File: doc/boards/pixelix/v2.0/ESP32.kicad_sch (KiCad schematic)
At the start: 2 parts, among them U1 ESP32-DEVKITC-32D

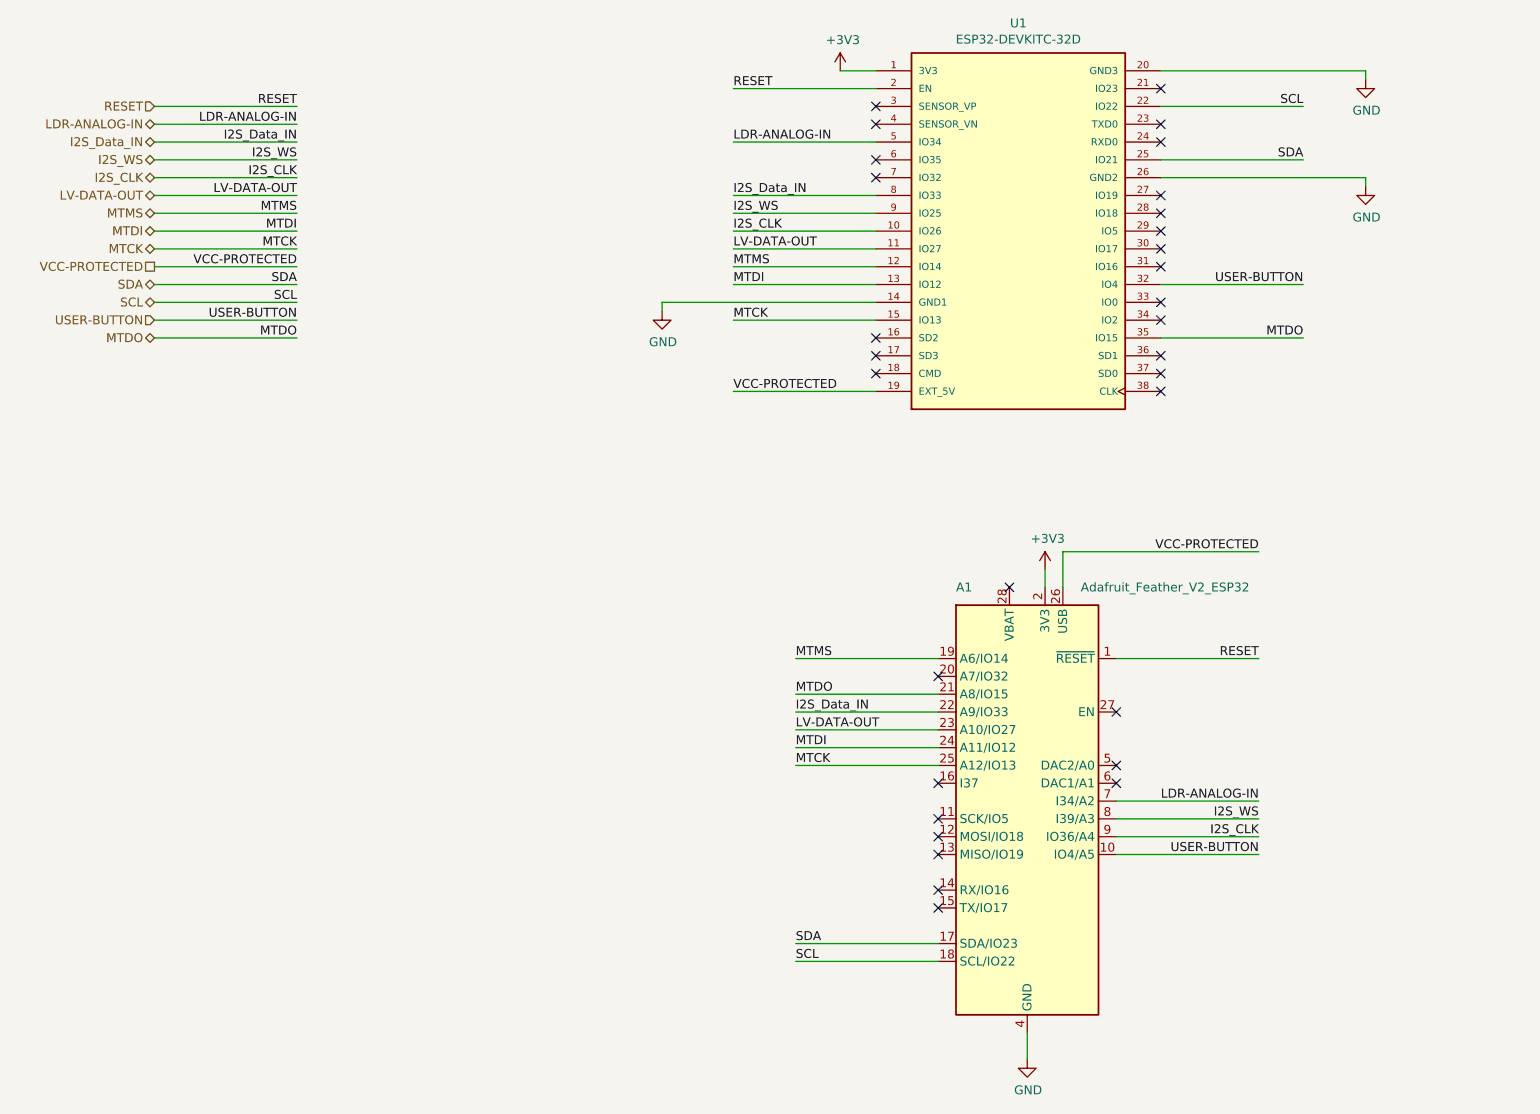
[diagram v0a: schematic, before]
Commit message: #91 Board v2.1 Schmatic - I2S Pins on Feather updated (see Table: https://github.com/BlueAndi/esp-rgb-led-matrix/blob/Development/doc/boards/pixelix/v2.0/ELECTRONIC.md)
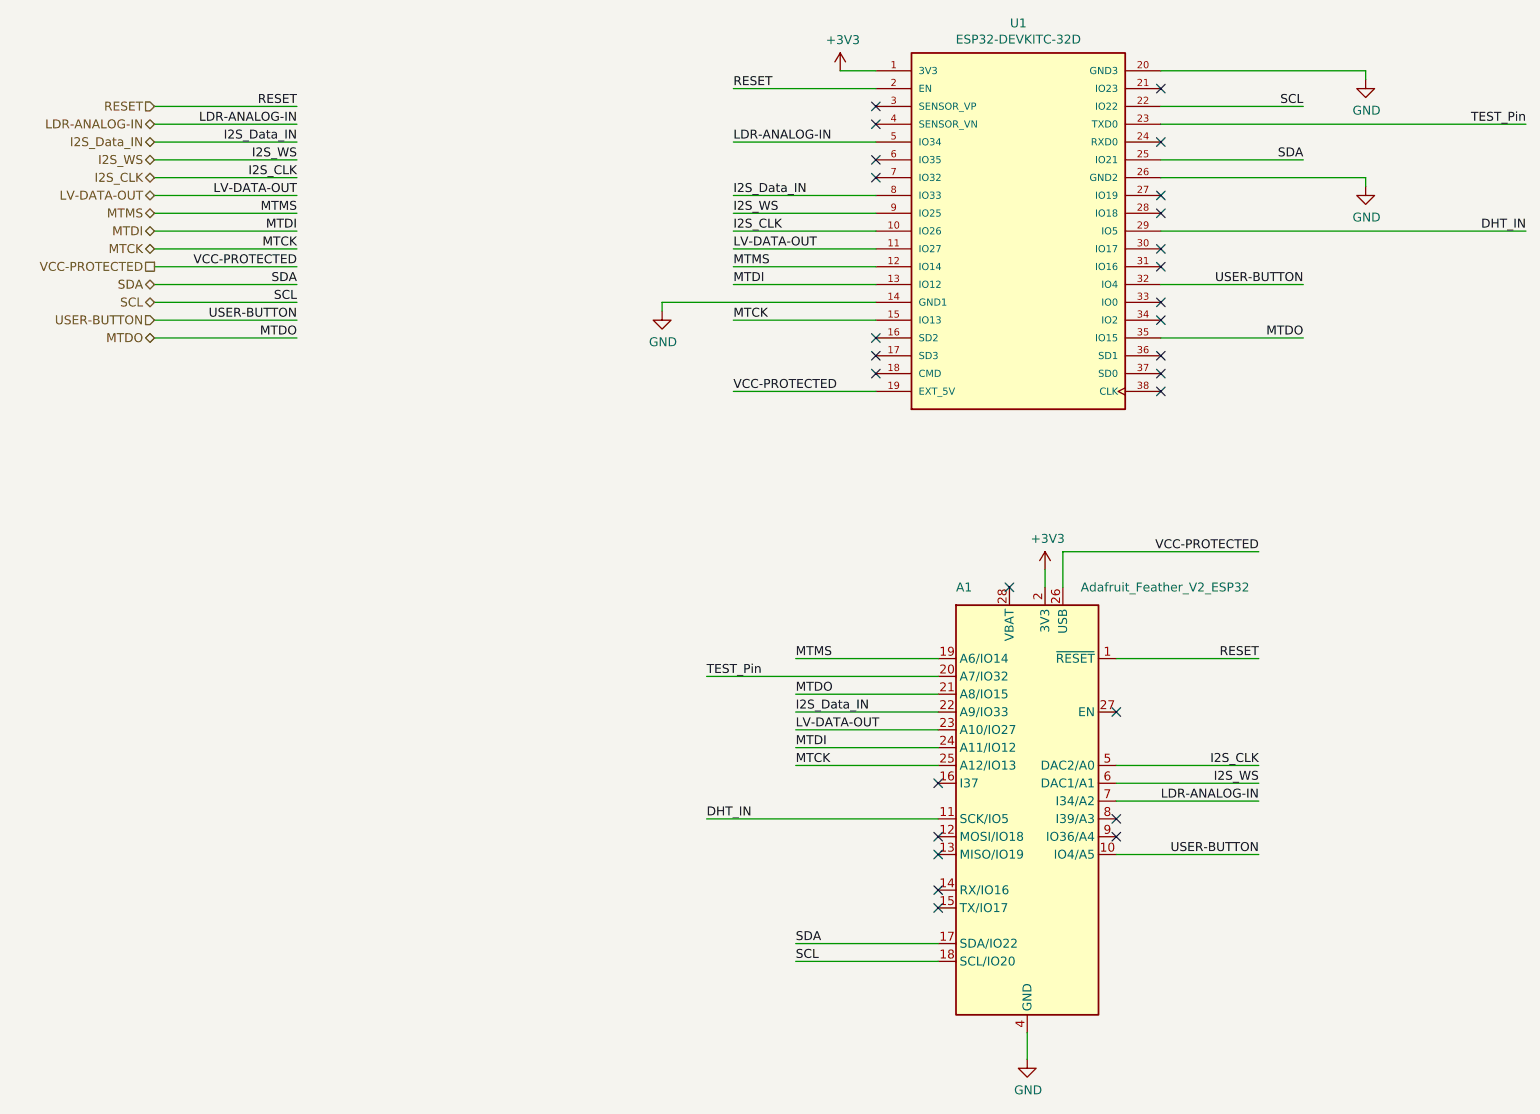
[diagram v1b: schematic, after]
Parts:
- A1: footprint footprints:Adafruit_Feather_V2_ESP32 -> Module:Adafruit_Feather
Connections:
- net I2S_CLK: now also A1.5 (DAC2/A0); no longer A1.9 (IO36/A4)
- net I2S_WS: now also A1.6 (DAC1/A1); no longer A1.8 (I39/A3)
- net TEST_Pin: now reaches U1.23 (TXD0)
- net TEST_Pin: now also A1.20 (A7/IO32)
- net DHT_IN: now reaches U1.29 (IO5)
- net DHT_IN: now also A1.11 (SCK/IO5)
- no-connect marks 31 -> 27
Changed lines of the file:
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@@
   (no_connect (at 139.7 30.48))
   (no_connect (at 180.34 66.04))
-  (no_connect (at 173.99 121.92))
-  (no_connect (at 173.99 124.46))
+  (no_connect (at 173.99 129.54))
+  (no_connect (at 173.99 132.08))
   (no_connect (at 180.34 55.88))
   (no_connect (at 139.7 60.96))
-  (no_connect (at 180.34 30.48))
   (no_connect (at 139.7 63.5))
   (no_connect (at 139.7 27.94))
   (no_connect (at 139.7 35.56))
-  (no_connect (at 148.59 109.22))
   (no_connect (at 180.34 48.26))
   (no_connect (at 148.59 124.46))
-  (no_connect (at 180.34 45.72))
   (no_connect (at 148.59 134.62))
-  (no_connect (at 148.59 129.54))
   (no_connect (at 148.59 142.24))
   (no_connect (at 180.34 43.18))
@@
     (stroke (width 0) (type default) (color 0 0 0 0))
   )
-  (wire (pts (xy 194.31 132.08) (xy 173.99 132.08))
+  (wire (pts (xy 194.31 121.92) (xy 173.99 121.92))
     (stroke (width 0) (type default) (color 0 0 0 0))
   )
@@
     (stroke (width 0) (type default) (color 0 0 0 0))
   )
+  (wire (pts (xy 115.57 129.54) (xy 148.59 129.54))
+    (stroke (width 0) (type default) (color 0 0 0 0))
+  )
+  (wire (pts (xy 115.57 109.22) (xy 148.59 109.22))
+    (stroke (width 0) (type default) (color 0 0 0 0))
+  )
   (wire (pts (xy 209.55 22.86) (xy 180.34 22.86))
     (stroke (width 0) (type default) (color 0 0 0 0))
@@
     (stroke (width 0) (type default) (color 0 0 0 0))
   )
-  (wire (pts (xy 194.31 129.54) (xy 173.99 129.54))
+  (wire (pts (xy 180.34 45.72) (xy 232.41 45.72))
+    (stroke (width 0) (type default) (color 0 0 0 0))
+  )
+  (wire (pts (xy 194.31 124.46) (xy 173.99 124.46))
+    (stroke (width 0) (type default) (color 0 0 0 0))
+  )
+  (wire (pts (xy 232.41 30.48) (xy 180.34 30.48))
     (stroke (width 0) (type default) (color 0 0 0 0))
   )
@@
     (effects (font (size 1.27 1.27)) (justify left bottom))
   )
-  (label "I2S_CLK" (at 194.31 132.08 180)
+  (label "I2S_CLK" (at 194.31 121.92 180)
     (effects (font (size 1.27 1.27)) (justify right bottom))
   )
@@
     (effects (font (size 1.27 1.27)) (justify left bottom))
   )
+  (label "TEST_Pin" (at 115.57 109.22 0)
+    (effects (font (size 1.27 1.27)) (justify left bottom))
+  )
   (label "LDR-ANALOG-IN" (at 57.15 30.48 180)
     (effects (font (size 1.27 1.27)) (justify right bottom))
   )
+  (label "DHT_IN" (at 232.41 45.72 180)
+    (effects (font (size 1.27 1.27)) (justify right bottom))
+  )
   (label "SDA" (at 128.27 147.32 0)
     (effects (font (size 1.27 1.27)) (justify left bottom))
@@
     (effects (font (size 1.27 1.27)) (justify right bottom))
   )
+  (label "TEST_Pin" (at 232.41 30.48 180)
+    (effects (font (size 1.27 1.27)) (justify right bottom))
+  )
   (label "MTCK" (at 119.38 58.42 0)
     (effects (font (size 1.27 1.27)) (justify left bottom))
@@
     (effects (font (size 1.27 1.27)) (justify right bottom))
   )
-  (label "I2S_WS" (at 194.31 129.54 180)
+  (label "I2S_WS" (at 194.31 124.46 180)
     (effects (font (size 1.27 1.27)) (justify right bottom))
   )
@@
   )
   (label "SCL" (at 128.27 149.86 0)
+    (effects (font (size 1.27 1.27)) (justify left bottom))
+  )
+  (label "DHT_IN" (at 115.57 129.54 0)
     (effects (font (size 1.27 1.27)) (justify left bottom))
   )
@@
       (effects (font (size 1.27 1.27)) (justify left))
     )
-    (property "Footprint" "footprints:Adafruit_Feather_V2_ESP32" (id 2) (at 163.83 161.29 0)
+    (property "Footprint" "Module:Adafruit_Feather" (id 2) (at 163.83 161.29 0)
       (effects (font (size 1.27 1.27)) (justify left) hide)
     )

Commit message: Revert "#91 Board v2.1 Schmatic"
This reverts commit 70677a910b1cfea4215dbaf6ed272a144c07ba06.
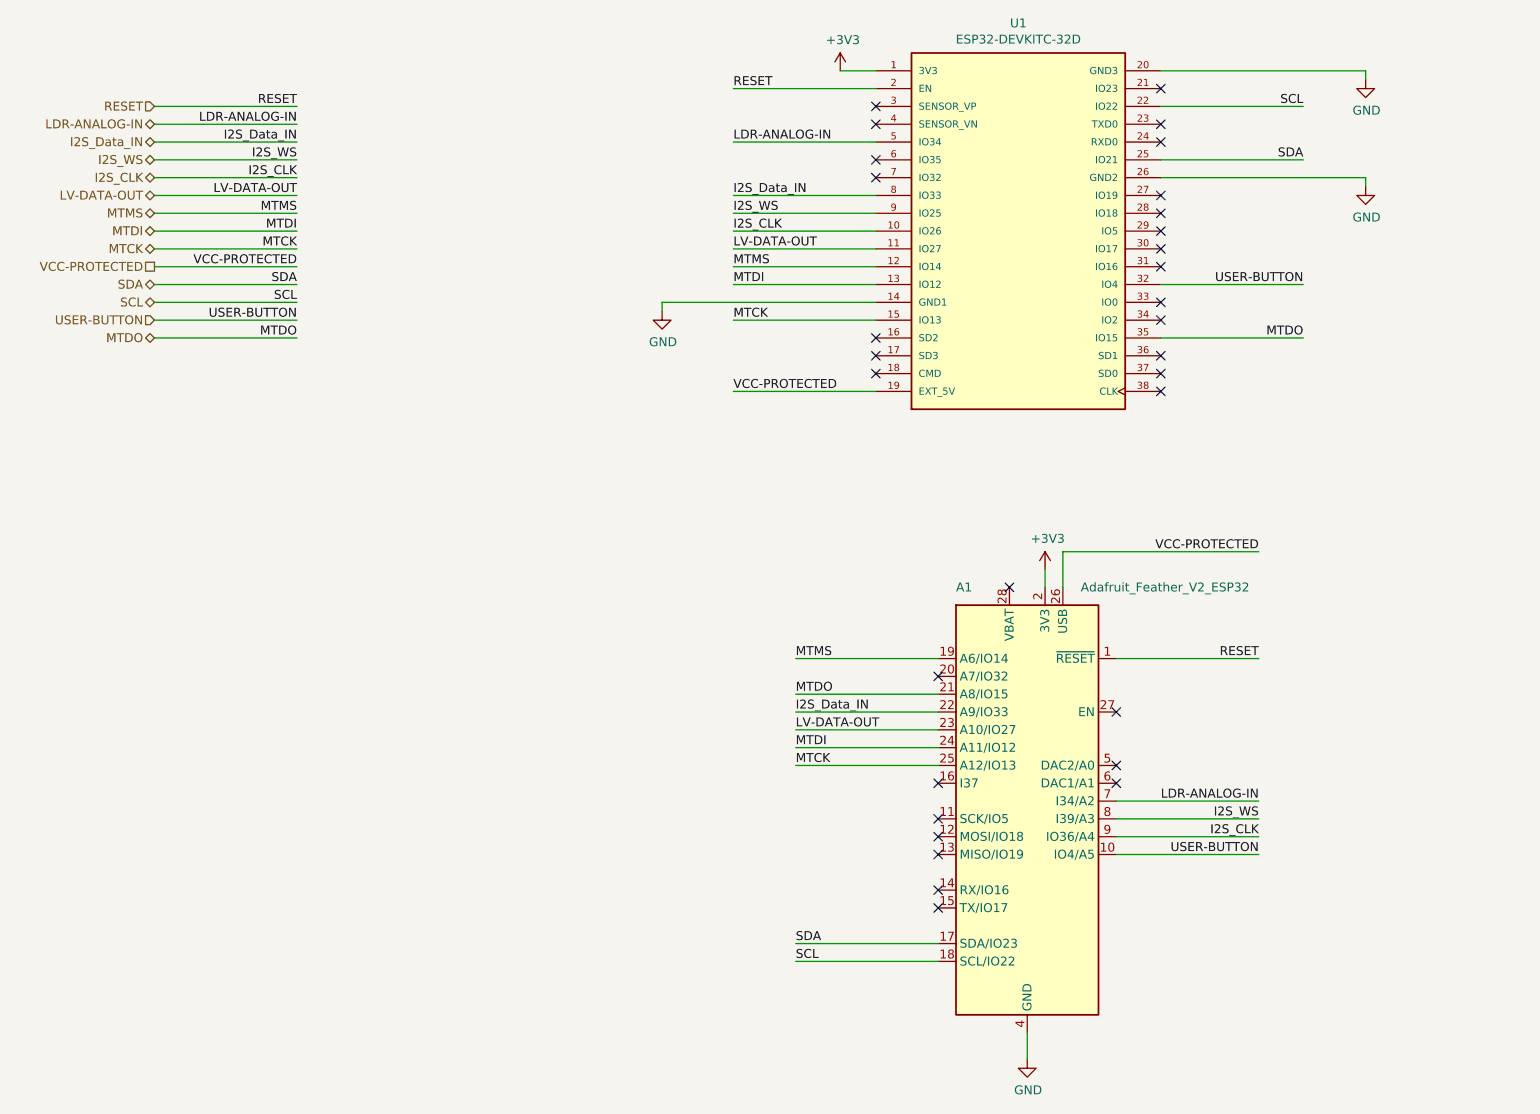
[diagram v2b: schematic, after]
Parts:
- A1: footprint Module:Adafruit_Feather -> footprints:Adafruit_Feather_V2_ESP32
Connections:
- net I2S_CLK: now also A1.9 (IO36/A4); no longer A1.5 (DAC2/A0)
- net I2S_WS: now also A1.8 (I39/A3); no longer A1.6 (DAC1/A1)
- net DHT_IN: no longer names the net of U1.29 (IO5)
- net DHT_IN: no longer A1.11 (SCK/IO5)
- net TEST_Pin: no longer names the net of U1.23 (TXD0)
- net TEST_Pin: no longer A1.20 (A7/IO32)
- no-connect marks 27 -> 31
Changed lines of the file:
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@@
   (no_connect (at 139.7 30.48))
   (no_connect (at 180.34 66.04))
-  (no_connect (at 173.99 129.54))
-  (no_connect (at 173.99 132.08))
+  (no_connect (at 173.99 121.92))
+  (no_connect (at 173.99 124.46))
   (no_connect (at 180.34 55.88))
   (no_connect (at 139.7 60.96))
+  (no_connect (at 180.34 30.48))
   (no_connect (at 139.7 63.5))
   (no_connect (at 139.7 27.94))
   (no_connect (at 139.7 35.56))
+  (no_connect (at 148.59 109.22))
   (no_connect (at 180.34 48.26))
   (no_connect (at 148.59 124.46))
+  (no_connect (at 180.34 45.72))
   (no_connect (at 148.59 134.62))
+  (no_connect (at 148.59 129.54))
   (no_connect (at 148.59 142.24))
   (no_connect (at 180.34 43.18))
@@
     (stroke (width 0) (type default) (color 0 0 0 0))
   )
-  (wire (pts (xy 194.31 121.92) (xy 173.99 121.92))
+  (wire (pts (xy 194.31 132.08) (xy 173.99 132.08))
     (stroke (width 0) (type default) (color 0 0 0 0))
   )
@@
     (stroke (width 0) (type default) (color 0 0 0 0))
   )
-  (wire (pts (xy 115.57 129.54) (xy 148.59 129.54))
-    (stroke (width 0) (type default) (color 0 0 0 0))
-  )
-  (wire (pts (xy 115.57 109.22) (xy 148.59 109.22))
-    (stroke (width 0) (type default) (color 0 0 0 0))
-  )
   (wire (pts (xy 209.55 22.86) (xy 180.34 22.86))
     (stroke (width 0) (type default) (color 0 0 0 0))
@@
     (stroke (width 0) (type default) (color 0 0 0 0))
   )
-  (wire (pts (xy 180.34 45.72) (xy 232.41 45.72))
-    (stroke (width 0) (type default) (color 0 0 0 0))
-  )
-  (wire (pts (xy 194.31 124.46) (xy 173.99 124.46))
-    (stroke (width 0) (type default) (color 0 0 0 0))
-  )
-  (wire (pts (xy 232.41 30.48) (xy 180.34 30.48))
+  (wire (pts (xy 194.31 129.54) (xy 173.99 129.54))
     (stroke (width 0) (type default) (color 0 0 0 0))
   )
@@
     (effects (font (size 1.27 1.27)) (justify left bottom))
   )
-  (label "I2S_CLK" (at 194.31 121.92 180)
+  (label "I2S_CLK" (at 194.31 132.08 180)
     (effects (font (size 1.27 1.27)) (justify right bottom))
   )
@@
     (effects (font (size 1.27 1.27)) (justify left bottom))
   )
-  (label "TEST_Pin" (at 115.57 109.22 0)
-    (effects (font (size 1.27 1.27)) (justify left bottom))
-  )
   (label "LDR-ANALOG-IN" (at 57.15 30.48 180)
     (effects (font (size 1.27 1.27)) (justify right bottom))
   )
-  (label "DHT_IN" (at 232.41 45.72 180)
-    (effects (font (size 1.27 1.27)) (justify right bottom))
-  )
   (label "SDA" (at 128.27 147.32 0)
     (effects (font (size 1.27 1.27)) (justify left bottom))
@@
     (effects (font (size 1.27 1.27)) (justify right bottom))
   )
-  (label "TEST_Pin" (at 232.41 30.48 180)
-    (effects (font (size 1.27 1.27)) (justify right bottom))
-  )
   (label "MTCK" (at 119.38 58.42 0)
     (effects (font (size 1.27 1.27)) (justify left bottom))
@@
     (effects (font (size 1.27 1.27)) (justify right bottom))
   )
-  (label "I2S_WS" (at 194.31 124.46 180)
+  (label "I2S_WS" (at 194.31 129.54 180)
     (effects (font (size 1.27 1.27)) (justify right bottom))
   )
@@
   )
   (label "SCL" (at 128.27 149.86 0)
-    (effects (font (size 1.27 1.27)) (justify left bottom))
-  )
-  (label "DHT_IN" (at 115.57 129.54 0)
     (effects (font (size 1.27 1.27)) (justify left bottom))
   )
@@
       (effects (font (size 1.27 1.27)) (justify left))
     )
-    (property "Footprint" "Module:Adafruit_Feather" (id 2) (at 163.83 161.29 0)
+    (property "Footprint" "footprints:Adafruit_Feather_V2_ESP32" (id 2) (at 163.83 161.29 0)
       (effects (font (size 1.27 1.27)) (justify left) hide)
     )
